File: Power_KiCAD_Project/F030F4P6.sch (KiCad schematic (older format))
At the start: 11 parts, among them U4 STM32F030F4P6, Y1 Crystal

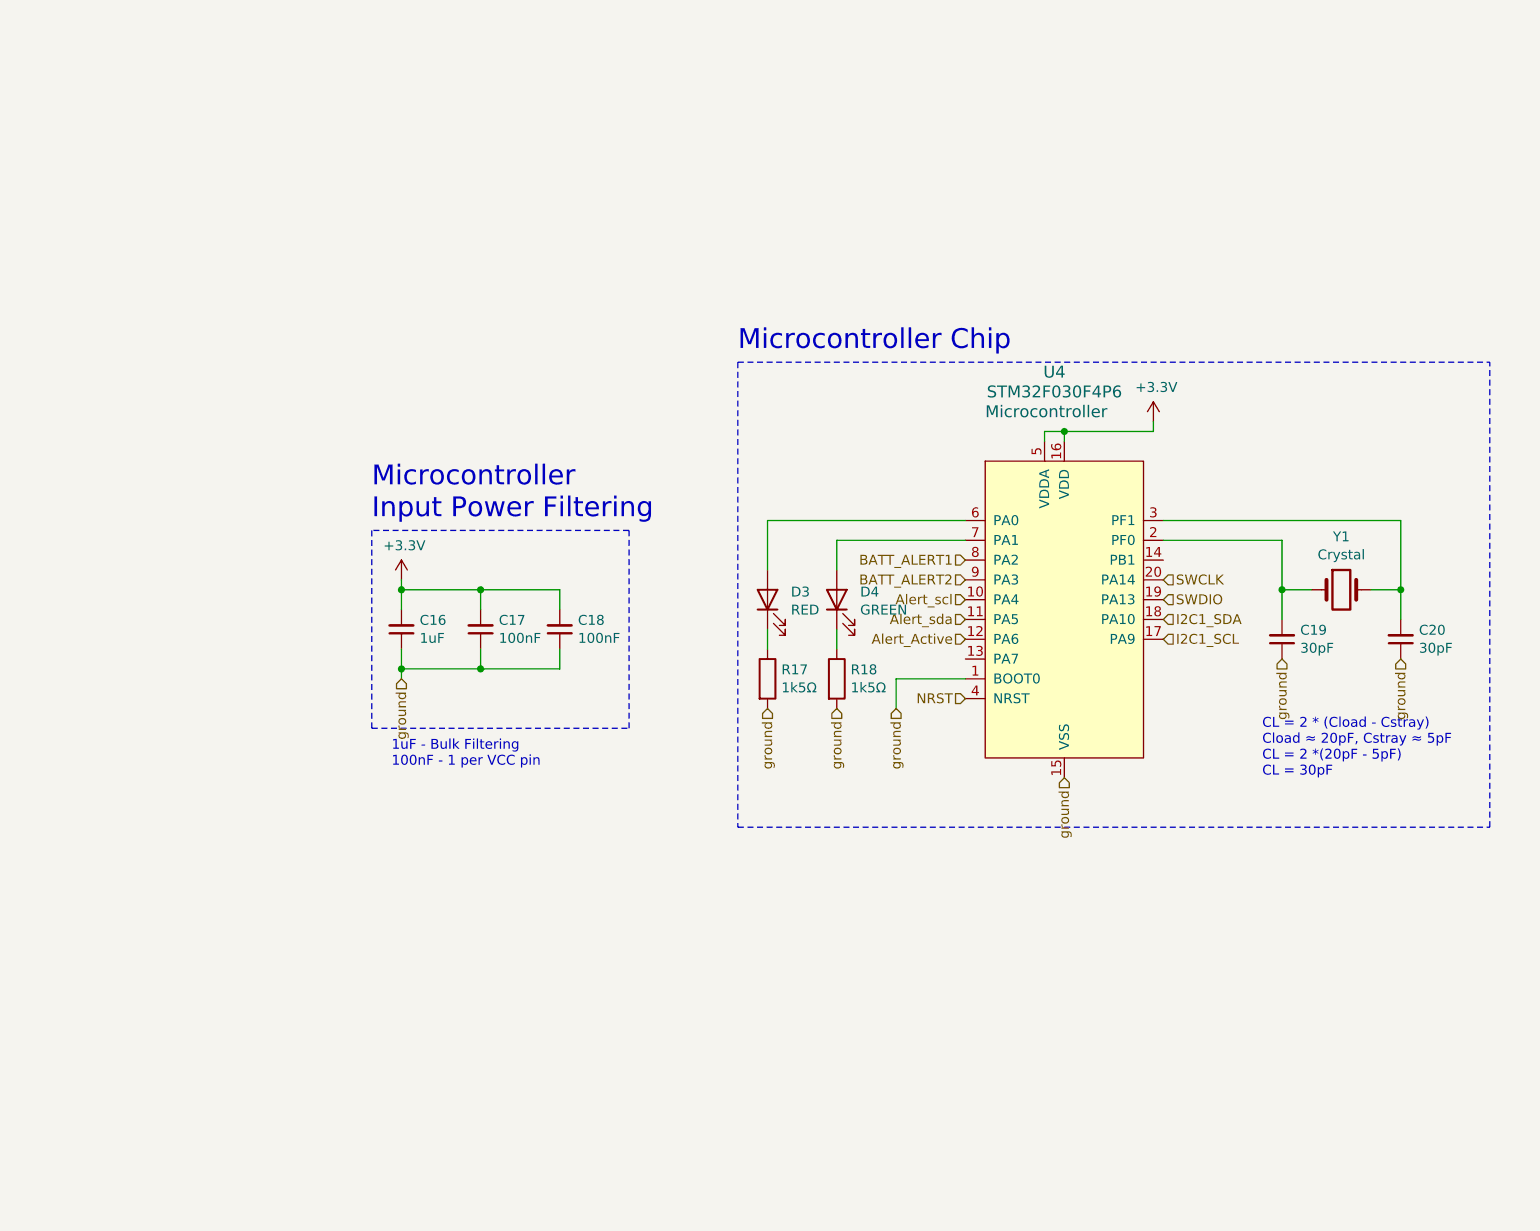
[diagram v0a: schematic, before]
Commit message: pcb finished
pcb is done. 3am kicad be like
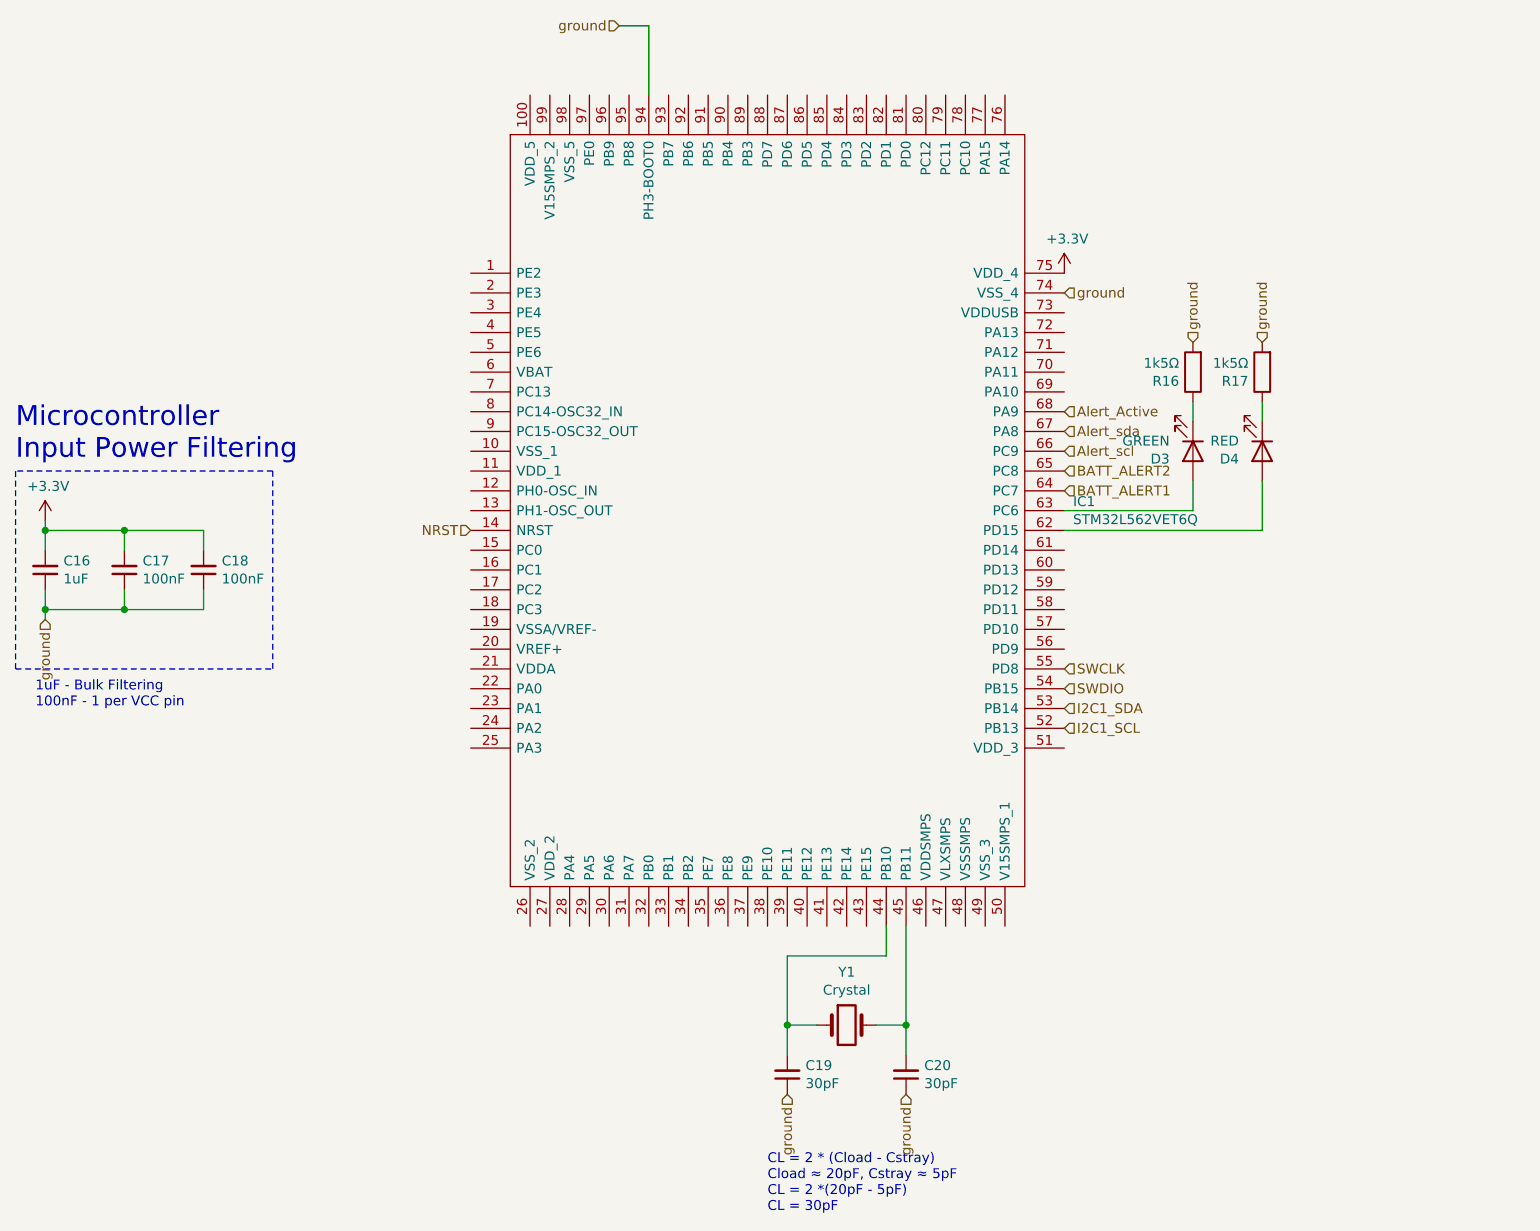
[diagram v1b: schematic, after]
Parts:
- removed U4: STM32F030F4P6, digikey-footprints:TSSOP-20_W4.4mm, symbol dk_Embedded-Microcontrollers:STM32F030F4P6
- added IC1: STM32L562VET6Q, SamacSys_Parts:QFP50P1600X1600X160-100N, symbol SamacSys_Parts:STM32L562VET6Q
- renumbered D4 to D3, D3 to D4, R18 to R16
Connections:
- net +3V3: now also IC1.75 (VDD_4)
- net Alert_Active: now also IC1.68 (PA9)
- net Alert_scl: now also IC1.66 (PC9)
- net Alert_sda: now also IC1.67 (PA8)
- net BATT_ALERT1: now also IC1.64 (PC7)
- net BATT_ALERT2: now also IC1.65 (PC8)
- net I2C1_SCL: now also IC1.52 (PB13)
- net I2C1_SDA: now also IC1.53 (PB14)
- net NRST: now also IC1.14 (NRST)
- net SWCLK: now also IC1.55 (PD8)
- net SWDIO: now also IC1.54 (PB15)
- net ground: now also IC1.74 (VSS_4), IC1.94 (PH3-BOOT0)
- net at C19.2, Y1.1: now also IC1.44 (PB10)
- net at C20.2, Y1.2: now also IC1.45 (PB11)
- net at D4.2 (A): now also IC1.62 (PD15)
- net at D3.2 (A): now also IC1.63 (PC6)
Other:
- note removed: "Microcontroller Chip"
- moved on the sheet: C16, C17, C18, C19, C20, D3, D4, R16, R17, Y1
